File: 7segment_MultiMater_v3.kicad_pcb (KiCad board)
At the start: 4 copper layers, 100 x 60.7 mm, 91 parts, among them J1 Conn_01x04_Socket, J2 GearPosition, P1 USB_C_Plug_USB2.0, Q1 IRLML6402, U1 SA10-21SRWA, U2 W25Q16JVUXIQ, U3 TB62706BF, U4 74HC595, U5 NJM12877F33, U6 MCP25625x-x-SS, U7 TM1637, U8 RP2040, Y1 12M, Y2 16M

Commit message: シルク追加
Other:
- board text added: "TIOちゃん予定地"
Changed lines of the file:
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@@
+		)
+	)
+	(gr_text "TIOちゃん予定地"
+		(at 82 66.2 0)
+		(layer "B.SilkS")
+		(effects
+			(font
+				(size 3 3)
+				(thickness 0.1)
+			)
+			(justify left bottom mirror)
 		)
 	)

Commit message: コメント追加
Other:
- board text added: "M5"
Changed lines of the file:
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@@
+	)
+	(gr_line
+		(start 153.67 26.96)
+		(end 148.2 32.43)
+		(stroke
+			(width 0.1)
+			(type default)
+		)
+		(layer "Cmts.User")
+	)
+	(gr_line
+		(start 148.2 32.43)
+		(end 148.2 27.92)
+		(stroke
+			(width 0.1)
+			(type default)
+		)
+		(layer "Cmts.User")
+	)
+	(gr_line
+		(start 152.9 32.43)
+		(end 148.2 32.43)
+		(stroke
+			(width 0.1)
+			(type default)
+		)
+		(layer "Cmts.User")
 	)
 	(gr_line
@@
 		)
 	)
+	(gr_text "M5"
+		(at 153.67 25.59 0)
+		(layer "Cmts.User")
+		(effects
+			(font
+				(size 3 3)
+				(thickness 0.15)
+			)
+			(justify left bottom)
+		)
+	)

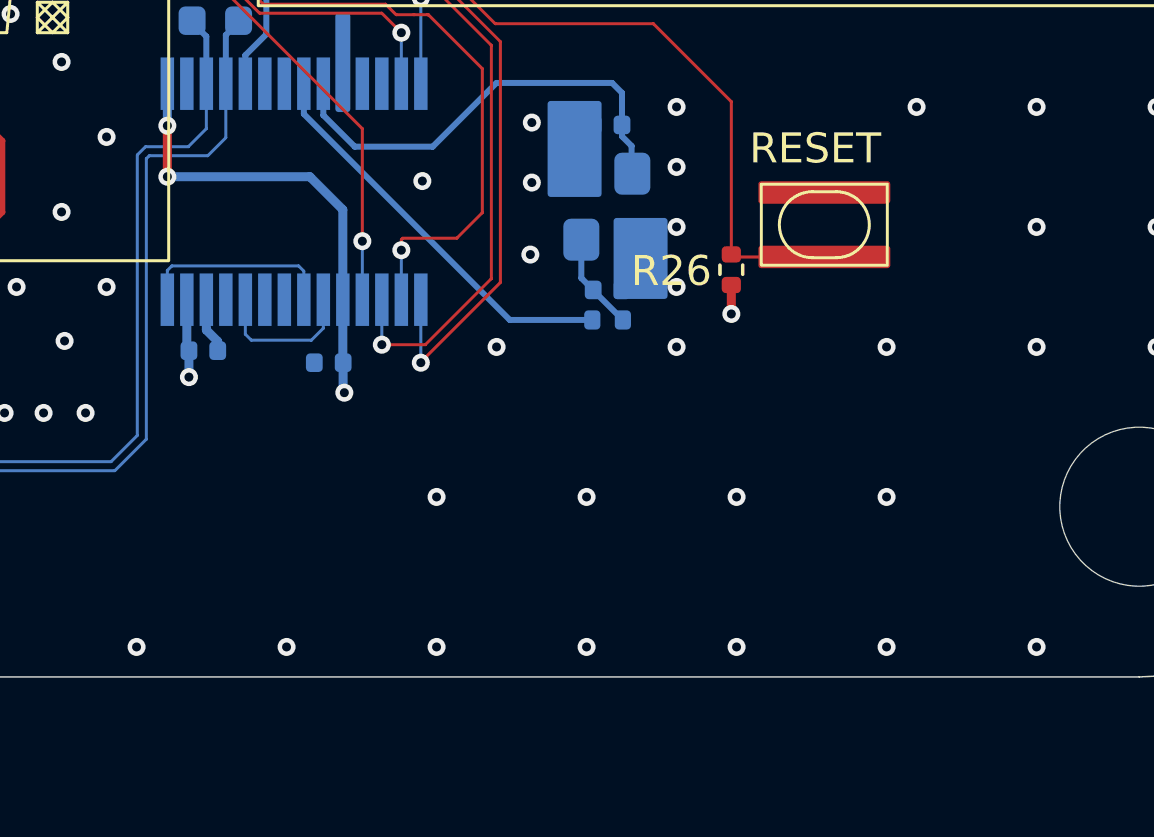
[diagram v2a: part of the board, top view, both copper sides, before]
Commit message: 微修正
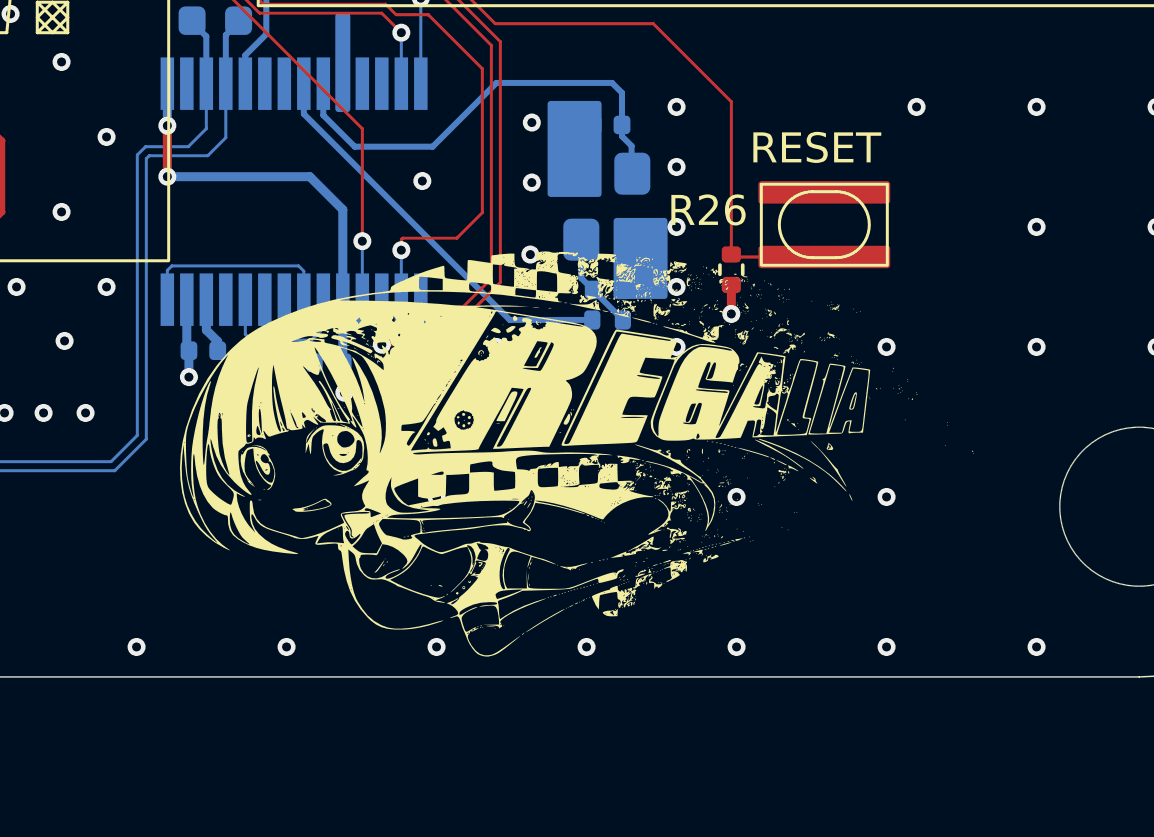
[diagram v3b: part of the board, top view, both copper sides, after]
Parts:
- added G***: LOGO, LOGO, F.Cu at (125.2, 85.2)
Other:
- board text removed: "TIOちゃん予定地"
